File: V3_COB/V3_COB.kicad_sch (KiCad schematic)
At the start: 2 parts, among them J101 Conn_02x35_Counter_Clockwise_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, J102 Conn_2Rows-76Pins

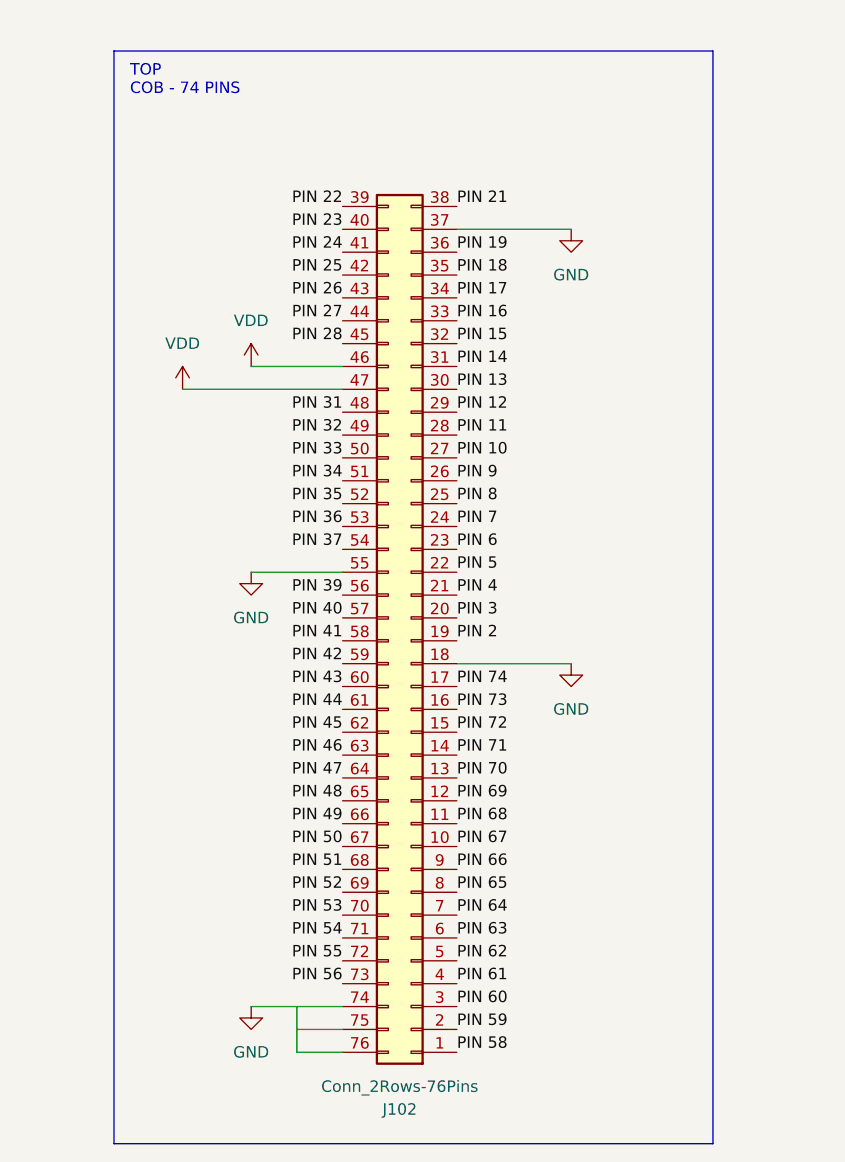
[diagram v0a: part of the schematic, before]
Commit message: XP update in V3_COB (clean up works)
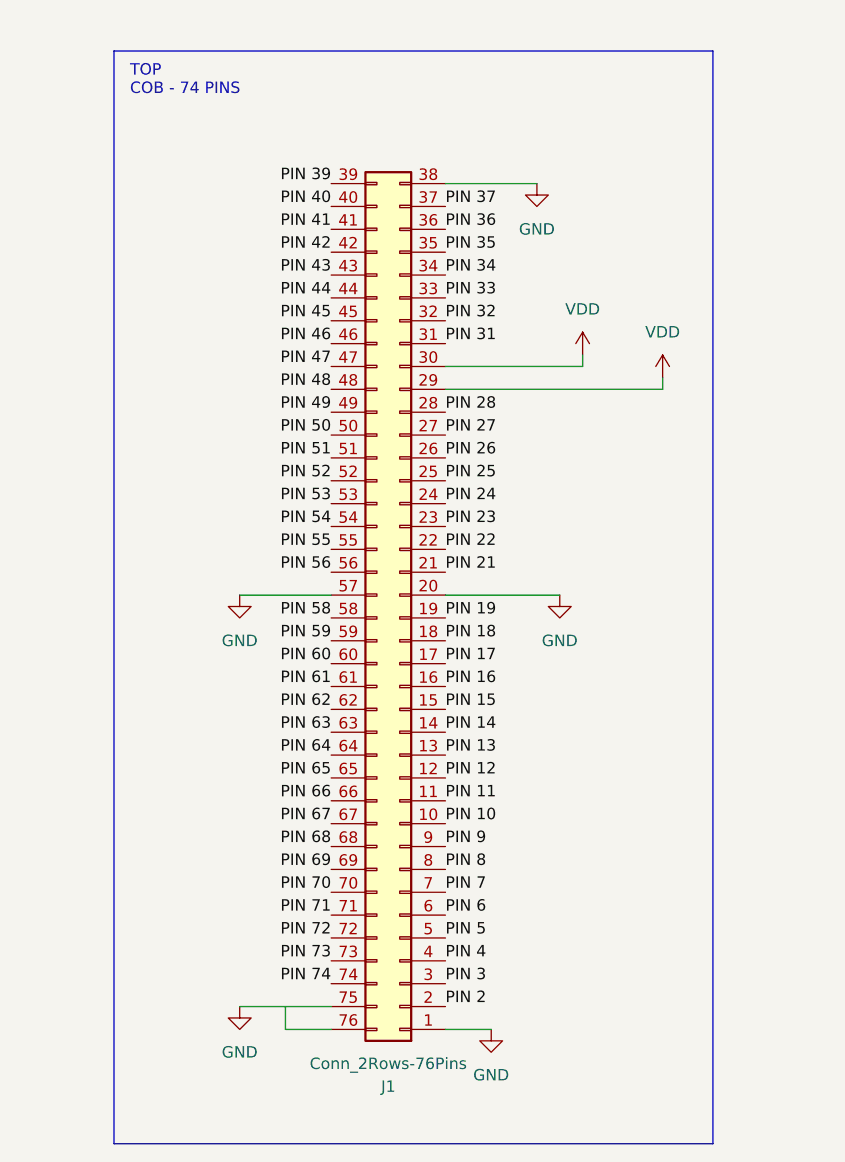
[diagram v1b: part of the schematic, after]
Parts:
- removed J102: Conn_2Rows-76Pins, MOSBius_V2_CHIP:round_COB, symbol Connector_Generic:Conn_02x38_Counter_Clockwise
- added J1: Conn_2Rows-76Pins, MOSBius_V2_CHIP:round_COB, symbol Connector_Generic:Conn_02x38_Counter_Clockwise
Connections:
- net GND: now also J1.1 (Pin_1), J1.20 (Pin_20), J1.38 (Pin_38), J1.57 (Pin_57), J1.75 (Pin_75)
- net PIN 10: now also J1.10 (Pin_10)
- net PIN 11: now also J1.11 (Pin_11)
- net PIN 12: now also J1.12 (Pin_12)
- net PIN 13: now also J1.13 (Pin_13)
- net PIN 14: now also J1.14 (Pin_14)
- net PIN 15: now also J1.15 (Pin_15)
- net PIN 16: now also J1.16 (Pin_16)
- net PIN 17: now also J1.17 (Pin_17)
- net PIN 18: now also J1.18 (Pin_18)
- net PIN 19: now also J1.19 (Pin_19)
- net PIN 2: now also J1.2 (Pin_2)
- net PIN 21: now also J1.21 (Pin_21)
- net PIN 22: now also J1.22 (Pin_22)
- net PIN 23: now also J1.23 (Pin_23)
- net PIN 24: now also J1.24 (Pin_24)
- net PIN 25: now also J1.25 (Pin_25)
- net PIN 26: now also J1.26 (Pin_26)
- net PIN 27: now also J1.27 (Pin_27)
- net PIN 28: now also J1.28 (Pin_28)
- net PIN 3: now also J1.3 (Pin_3)
- net PIN 31: now also J1.31 (Pin_31)
- net PIN 32: now also J1.32 (Pin_32)
- net PIN 33: now also J1.33 (Pin_33)
- net PIN 34: now also J1.34 (Pin_34)
- net PIN 35: now also J1.35 (Pin_35)
- net PIN 36: now also J1.36 (Pin_36)
- net PIN 37: now also J1.37 (Pin_37)
- net PIN 39: now also J1.39 (Pin_39)
- net PIN 4: now also J1.4 (Pin_4)
- net PIN 40: now also J1.40 (Pin_40)
- net PIN 41: now also J1.41 (Pin_41)
- net PIN 42: now also J1.42 (Pin_42)
- net PIN 43: now also J1.43 (Pin_43)
- net PIN 44: now also J1.44 (Pin_44)
- net PIN 45: now also J1.45 (Pin_45)
- net PIN 46: now also J1.46 (Pin_46)
- net PIN 47: now also J1.47 (Pin_47)
- net PIN 48: now also J1.48 (Pin_48)
- net PIN 49: now also J1.49 (Pin_49)
- net PIN 5: now also J1.5 (Pin_5)
- net PIN 50: now also J1.50 (Pin_50)
- net PIN 51: now also J1.51 (Pin_51)
- net PIN 52: now also J1.52 (Pin_52)
- net PIN 53: now also J1.53 (Pin_53)
- net PIN 54: now also J1.54 (Pin_54)
- net PIN 55: now also J1.55 (Pin_55)
- net PIN 56: now also J1.56 (Pin_56)
- net PIN 58: now also J1.58 (Pin_58)
- net PIN 59: now also J1.59 (Pin_59)
- net PIN 6: now also J1.6 (Pin_6)
- net PIN 60: now also J1.60 (Pin_60)
- net PIN 61: now also J1.61 (Pin_61)
- net PIN 62: now also J1.62 (Pin_62)
- net PIN 63: now also J1.63 (Pin_63)
- net PIN 64: now also J1.64 (Pin_64)
- net PIN 65: now also J1.65 (Pin_65)
- net PIN 66: now also J1.66 (Pin_66)
- net PIN 67: now also J1.67 (Pin_67)
- net PIN 68: now also J1.68 (Pin_68)
- net PIN 69: now also J1.69 (Pin_69)
- net PIN 7: now also J1.7 (Pin_7)
- net PIN 70: now also J1.70 (Pin_70)
- net PIN 71: now also J1.71 (Pin_71)
- net PIN 72: now also J1.72 (Pin_72)
- net PIN 73: now also J1.73 (Pin_73)
- net PIN 74: now also J1.74 (Pin_74)
- net PIN 8: now also J1.8 (Pin_8)
- net PIN 9: now also J1.9 (Pin_9)
- net VDD: now also J1.29 (Pin_29), J1.30 (Pin_30)
